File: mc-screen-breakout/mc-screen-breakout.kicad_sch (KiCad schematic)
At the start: 27 parts, among them J1 USB_C_Receptacle_PowerOnly_6P, J2 FH28-10S-0.5SH_05_, SW1 NANOT160BP, SW2 NANOT160BP, U1 CMM-3424DT-26165-TR, U2 MDBT50Q-1MV2, Y1 32.768kHz

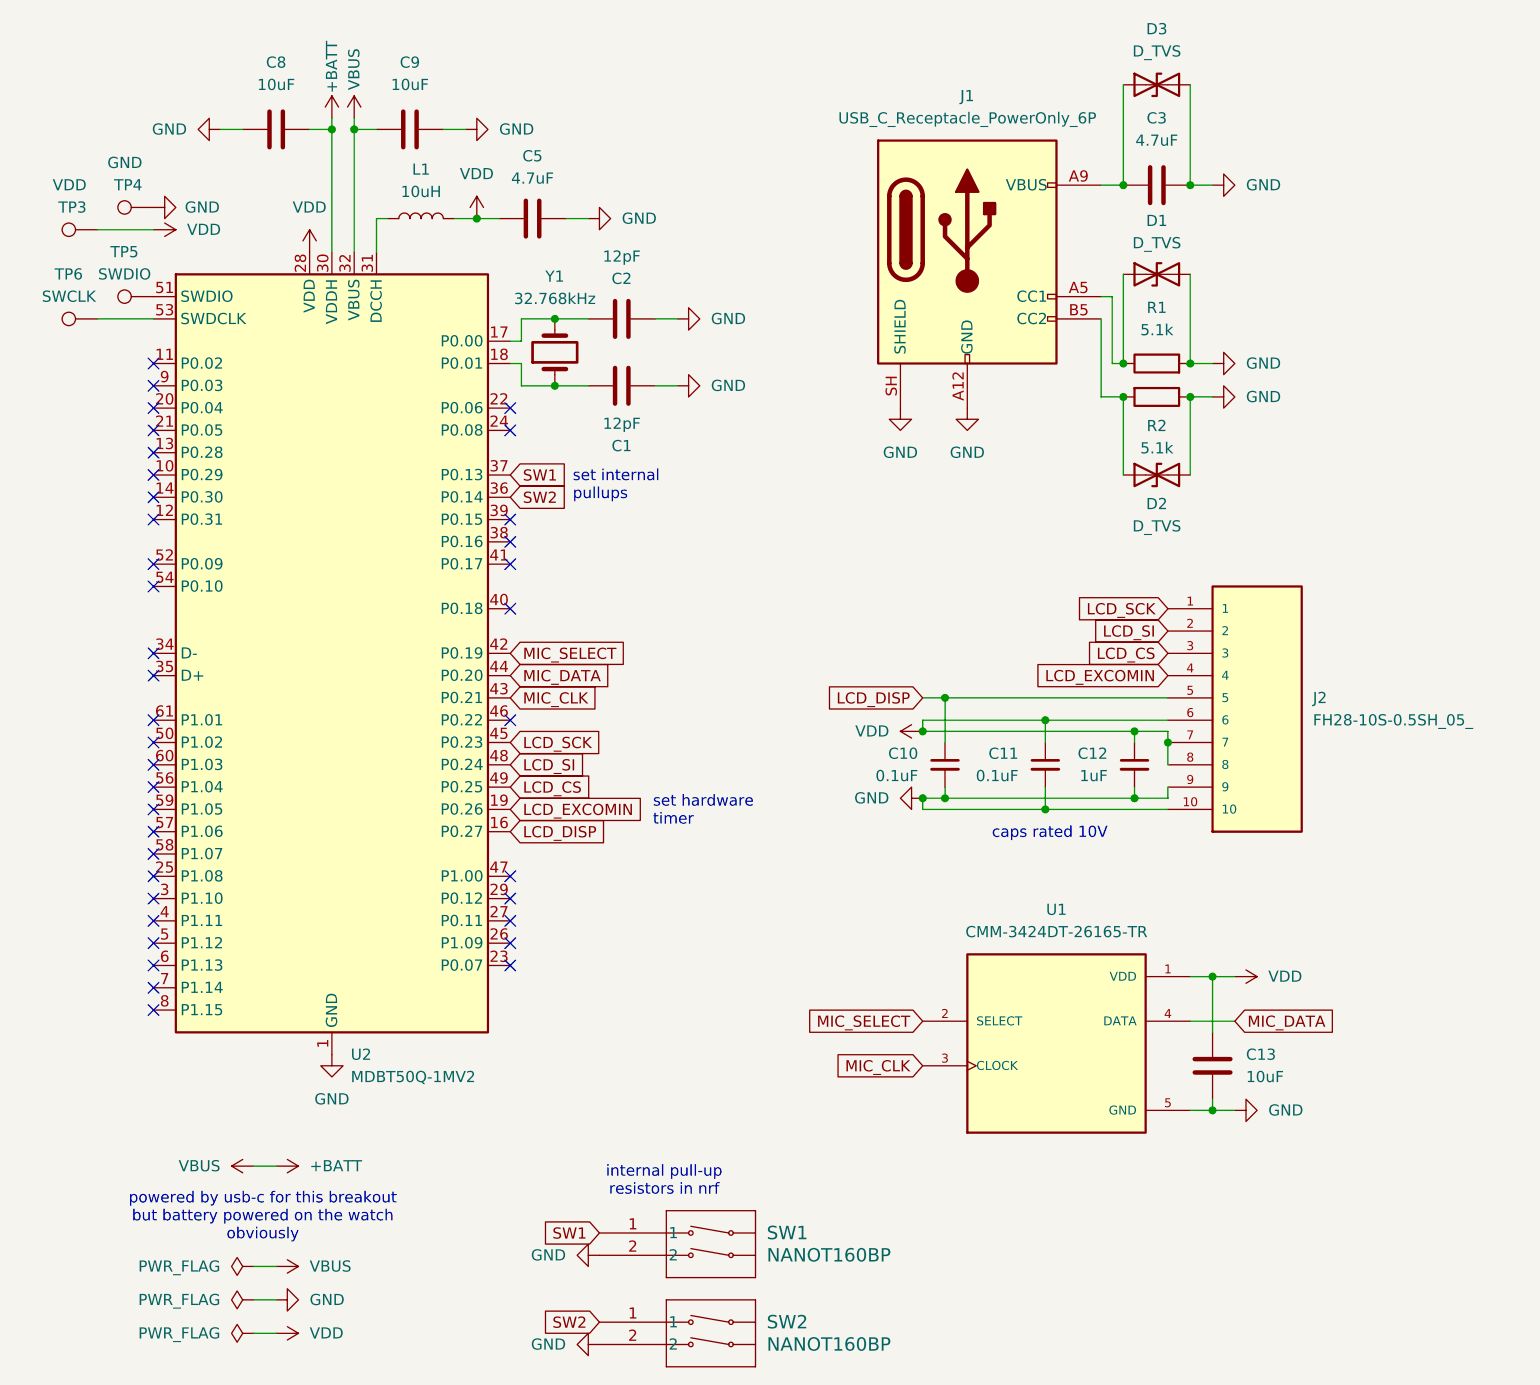
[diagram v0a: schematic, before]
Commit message: Began drawing traces
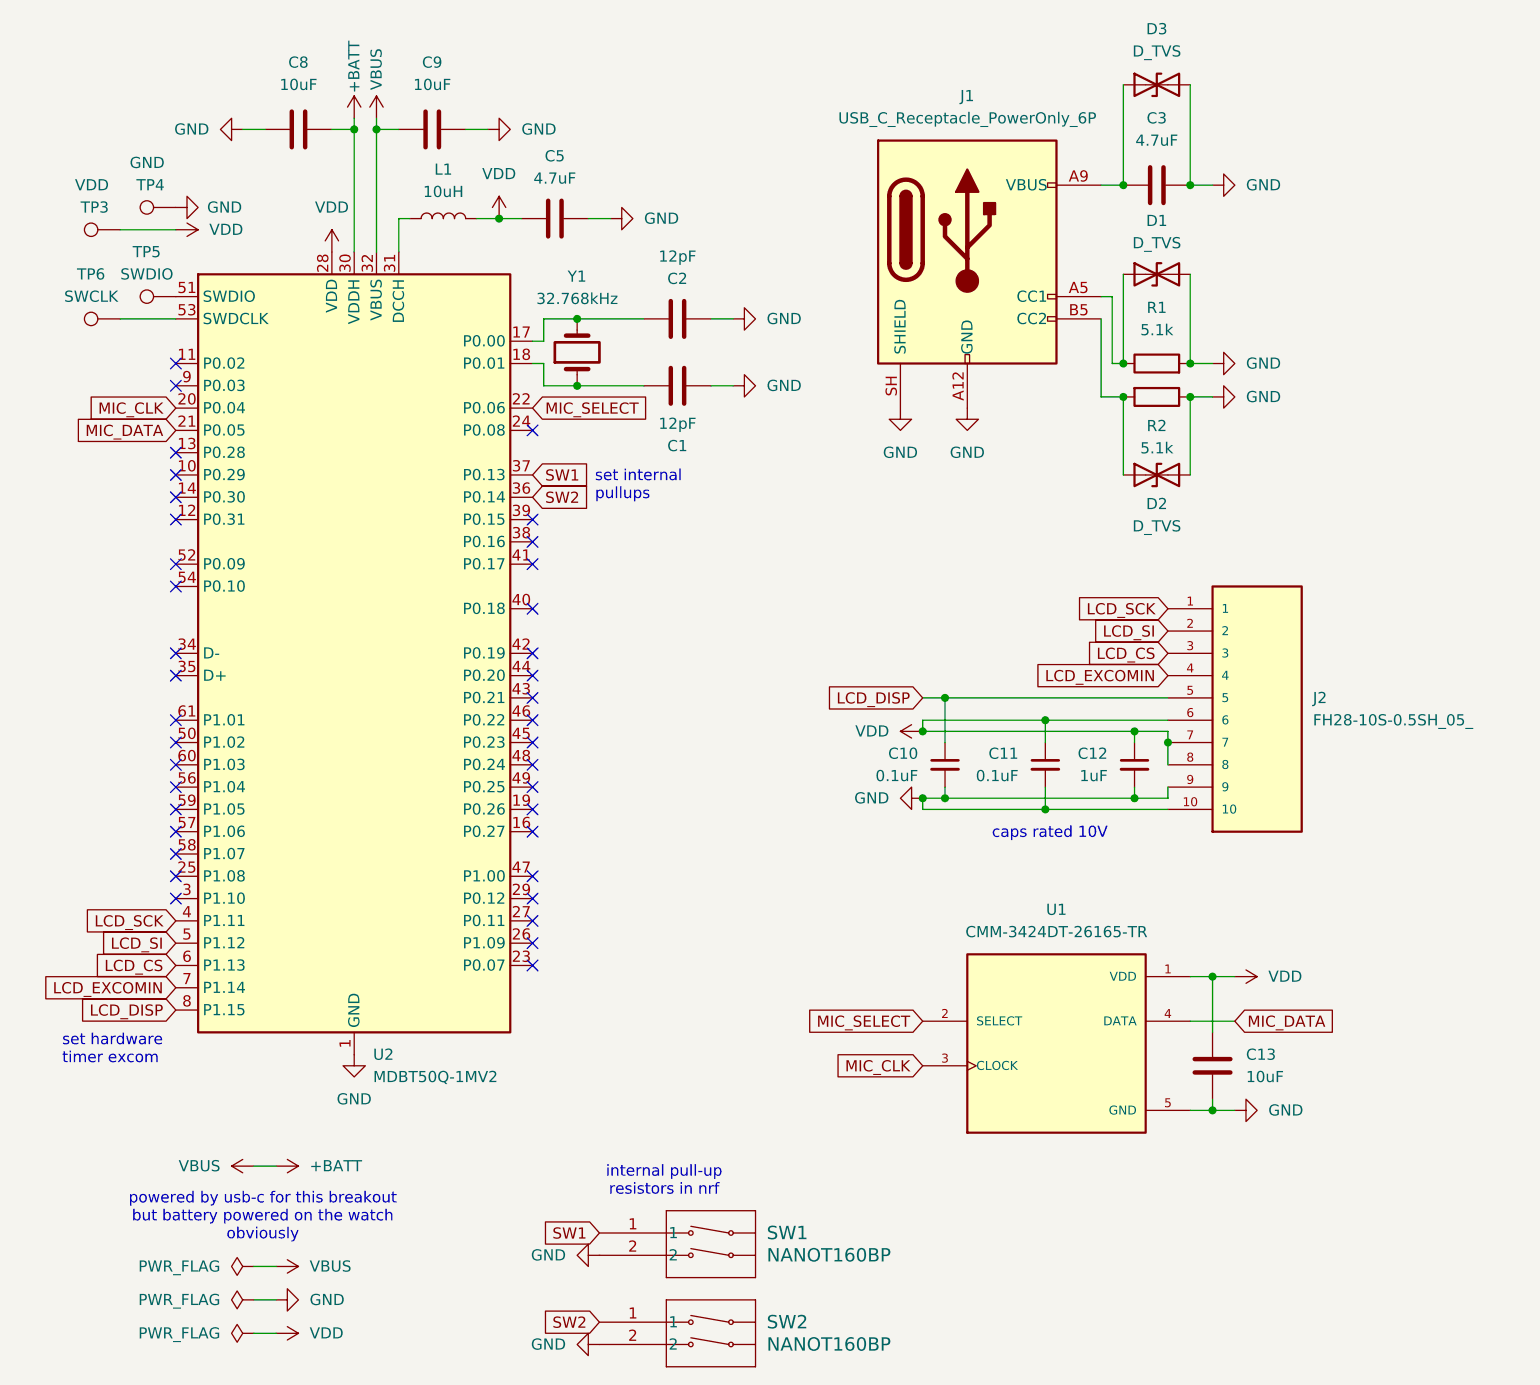
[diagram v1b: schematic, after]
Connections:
- net LCD_CS: now also U2.6 (P1.13); no longer U2.49 (P0.25)
- net LCD_DISP: now also U2.8 (P1.15); no longer U2.16 (P0.27)
- net LCD_EXCOMIN: now also U2.7 (P1.14); no longer U2.19 (P0.26)
- net LCD_SCK: now also U2.4 (P1.11); no longer U2.45 (P0.23)
- net LCD_SI: now also U2.5 (P1.12); no longer U2.48 (P0.24)
- net MIC_CLK: now also U2.20 (P0.04); no longer U2.43 (P0.21)
- net MIC_DATA: now also U2.21 (P0.05); no longer U2.44 (P0.20)
- net MIC_SELECT: now also U2.22 (P0.06); no longer U2.42 (P0.19)
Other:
- note added: "set hardware timer excom"
- note removed: "set hardware timer"
- moved on the sheet: C1, C2, C5, C8, C9, L1, TP3, TP4, TP5, TP6, U2, Y1
